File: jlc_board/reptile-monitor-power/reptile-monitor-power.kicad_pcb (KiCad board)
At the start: 4 copper layers, 38.1 x 53.3 mm, 14 parts, among them J1 AC_IN, J2 LOAD_2, J3 LOAD_1, J4 POWER CONN, K1 ALDP105W, K2 ALDP105W, U1 NUD3105DMT1G

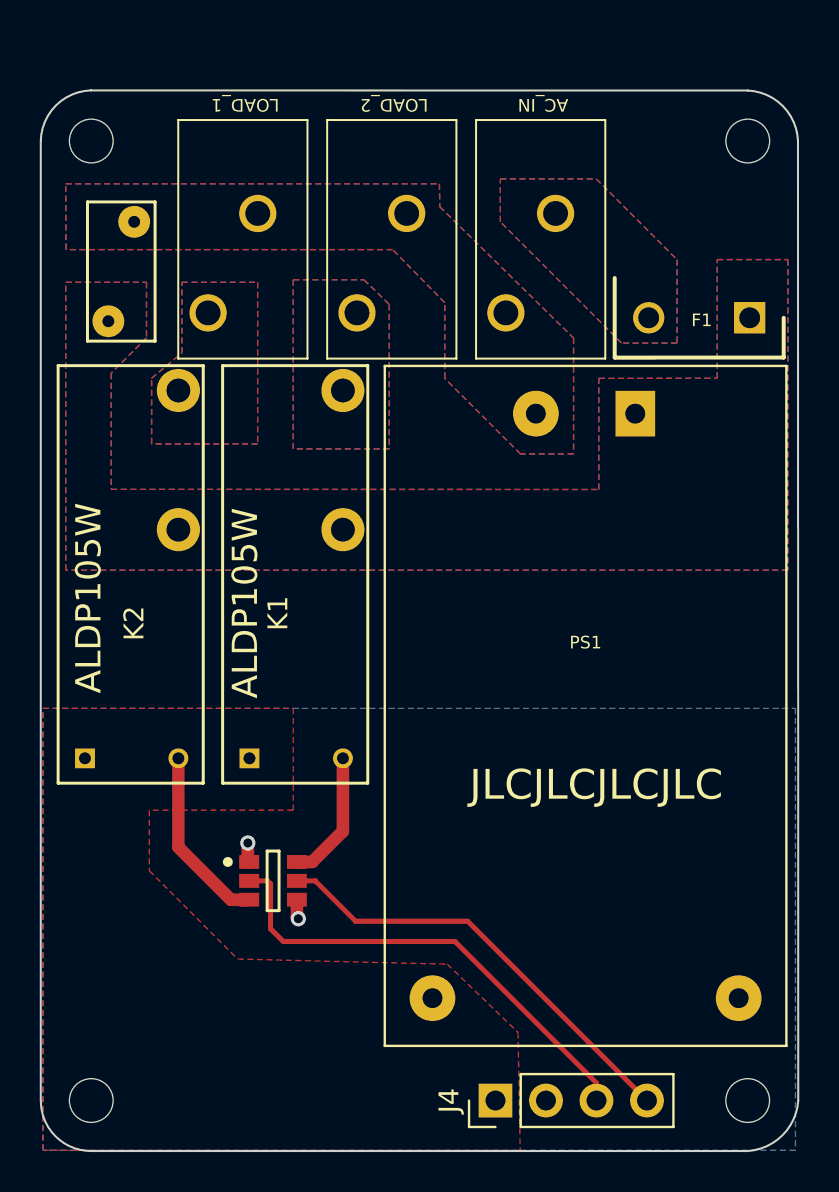
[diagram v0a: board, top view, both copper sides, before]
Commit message: rev4
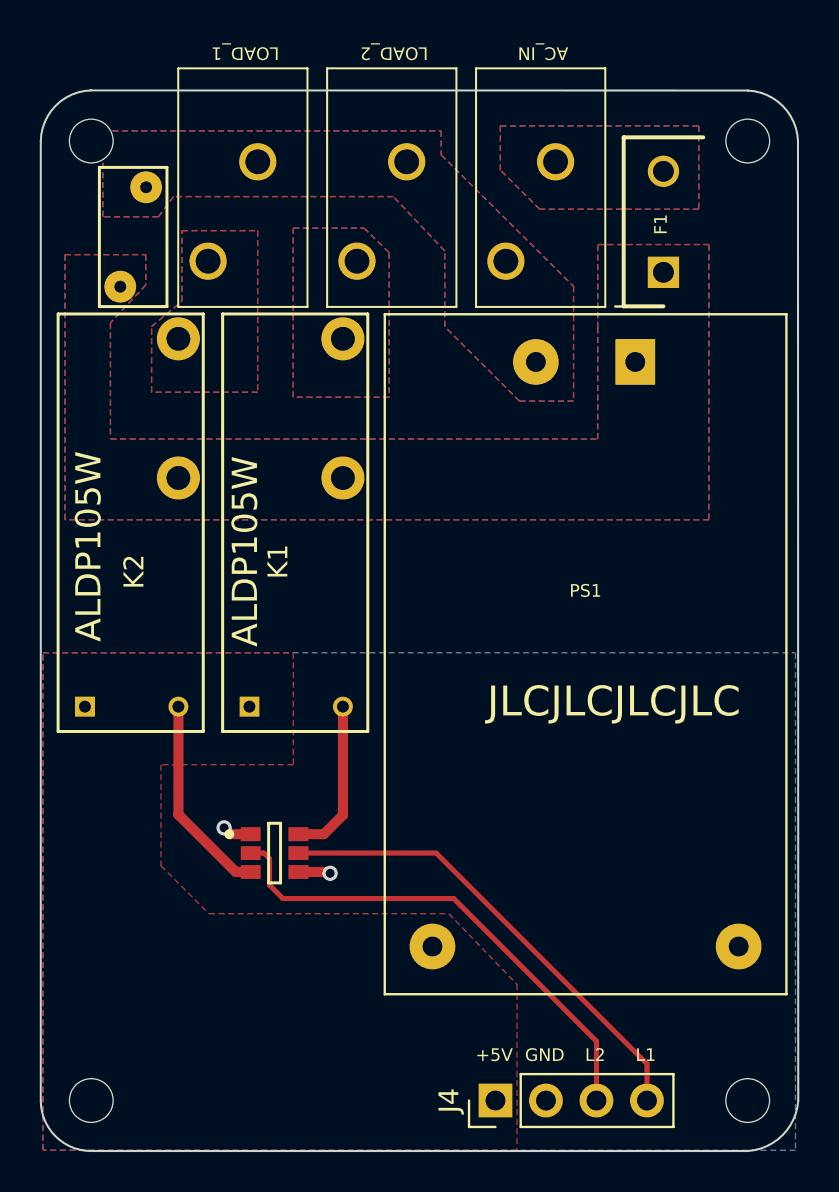
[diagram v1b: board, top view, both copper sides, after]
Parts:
- added REF**: WAFFLE, reptile-monitor:LOGO, B.Cu at (152.7, 83.9)
- J1, J2, J3: footprint reptile-monitor-power1:TE Connectivity PC Terminal Block 128340212 -> reptile-monitor-power:TE Connectivity PC Terminal Block 128340212
- RV1: footprint reptile-monitor-power1:RV_Disc_D7mm_W3.4mm_P5mm -> reptile-monitor-power:RV_Disc_D7mm_W3.4mm_P5mm
- moved F1 4.90 mm to (158.3, 59.9), turned to 90 degrees
- moved J1 2.60 mm to (152.9, 54.4)
- moved K1 2.60 mm to (137.5, 81.8)
- moved K2 2.60 mm to (129.2, 81.8)
- moved PS1 2.60 mm to (156.9, 64.5)
- moved J2 2.60 mm to (145.4, 54.4)
- moved J3 2.60 mm to (137.9, 54.4)
- moved RV1 1.84 mm to (132.3, 55.7)
- moved U1 1.40 mm to (138.8, 89.2)
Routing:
- net L1: track 22.2 -> 23.8 mm
- net RLY2: track 6.62 -> 8.09 mm
- net L2: track 23.9 -> 25.1 mm
- net RLY1: track 9.13 -> 10.3 mm
- net GND: track 1.97 -> 3.09 mm
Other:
- rule pad_to_mask_clearance: 0.0508 -> 0
- board text added: "+5V"
- board text added: "GND"
- board text added: "L1"
- board text added: "L2"
- board text added: "Rev. 4, Aug 2021"
- board text removed: "Rev. 3, July 2021"
